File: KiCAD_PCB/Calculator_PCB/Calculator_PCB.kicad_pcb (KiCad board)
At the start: 2 copper layers, 108 parts, among them J1 USB_B_Micro, SW1 SW_SPST, SW10 SW_SPST, SW11 SW_SPST, SW12 SW_SPST, SW13 SW_SPST, SW14 SW_SPST, SW15 SW_SPST, SW16 SW_SPST, SW17 SW_SPST, SW18 SW_SPST, SW19 SW_SPST, SW2 SW_SPST, SW20 SW_SPST, SW21 SW_SPST, SW22 SW_SPST, SW23 SW_SPST, SW24 SW_SPST, SW25 SW_SPST, SW26 SW_SPST, SW27 SW_SPST, SW28 SW_SPST, SW29 SW_SPST, SW3 SW_SPST, SW30 SW_SPST, SW31 SW_SPST, SW32 SW_SPST, SW33 SW_SPST, SW34 SW_SPST, SW35 SW_SPST, SW36 SW_SPST, SW37 SW_SPST, SW38 SW_SPST, SW39 SW_SPST, SW4 SW_SPST, SW40 SW_SPST, SW5 SW_SPST, SW6 SW_SPST, SW7 SW_SPST, SW8 SW_SPST, SW9 SW_SPST, U1 W25Q128JVS, U2 RP2040, U3 NCP1117-3.3_SOT223, Y1 ABLS-12.000MHZ-B4-T

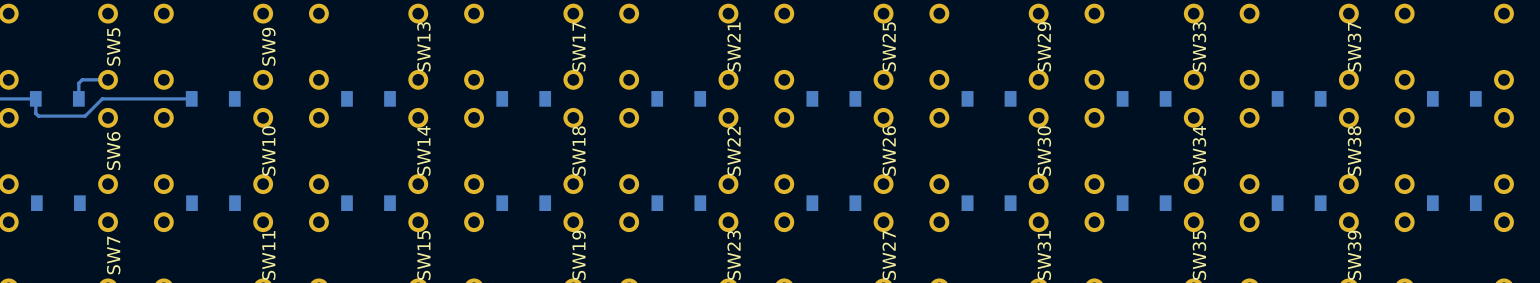
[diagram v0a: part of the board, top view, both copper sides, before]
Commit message: PCB Updates
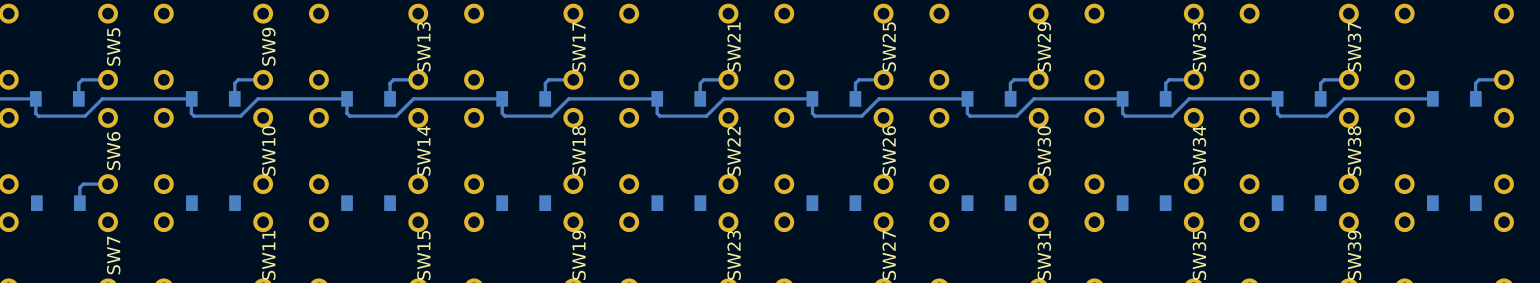
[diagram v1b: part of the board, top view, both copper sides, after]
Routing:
- net /Row0: track 17.6 -> 127.3 mm
- net Net-(D29-Pad2): track 0.00 -> 3.55 mm
- net Net-(D9-Pad2): track 0.00 -> 3.55 mm
- net Net-(D37-Pad2): track 0.00 -> 3.55 mm
- net Net-(D33-Pad2): track 0.00 -> 3.55 mm
- net Net-(D21-Pad2): track 0.00 -> 3.55 mm
- net Net-(D17-Pad2): track 0.00 -> 3.55 mm
- net Net-(D13-Pad2): track 0.00 -> 3.55 mm
- net Net-(D2-Pad2): track 0.00 -> 3.55 mm
- net Net-(D5-Pad2): track 0.00 -> 3.55 mm
- net Net-(D25-Pad2): track 0.00 -> 3.55 mm

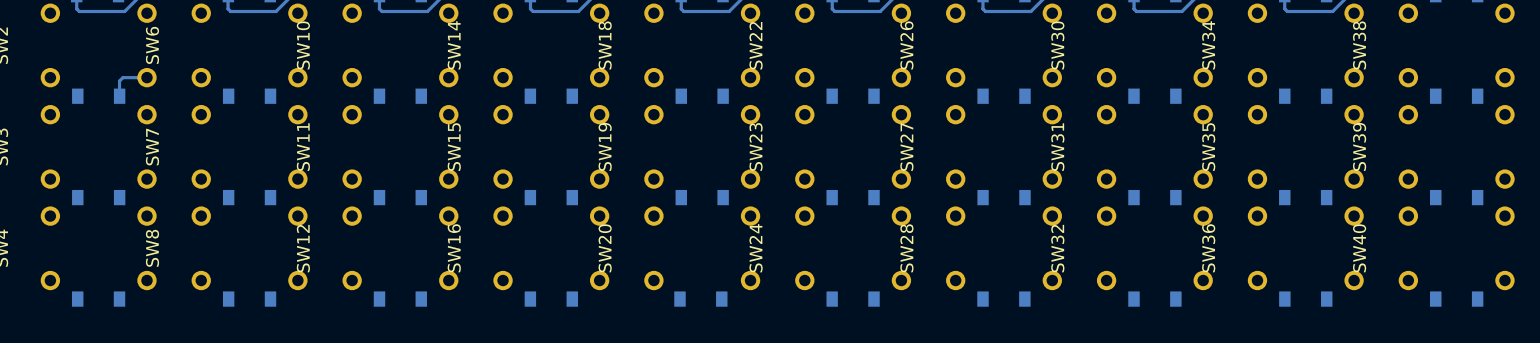
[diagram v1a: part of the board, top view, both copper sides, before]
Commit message: PCB Updates
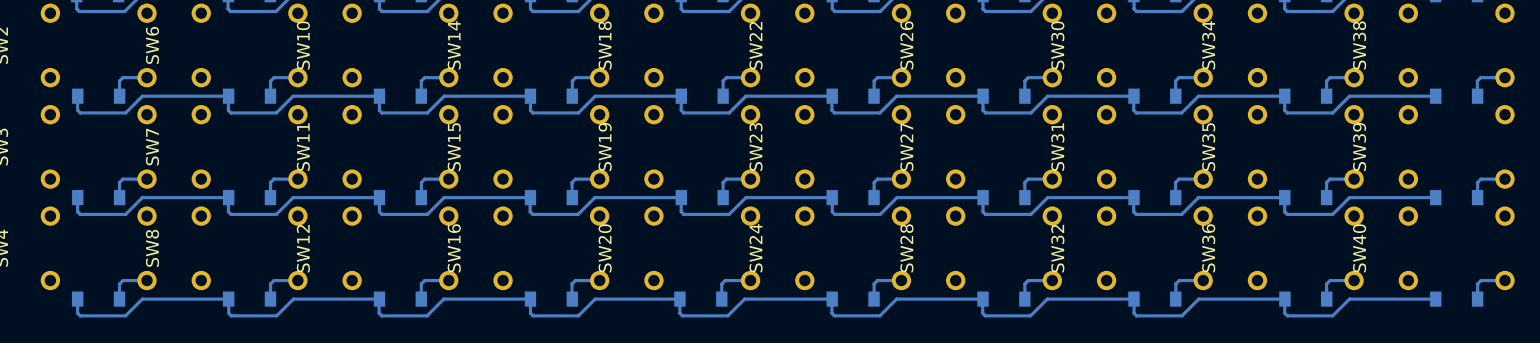
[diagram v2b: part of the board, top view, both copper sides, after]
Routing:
- net /Row3: track 0.00 -> 123.4 mm
- net /Row1: track 0.00 -> 123.4 mm
- net /Row2: track 0.00 -> 123.4 mm
- net Net-(D15-Pad2): track 0.00 -> 3.55 mm
- net Net-(D7-Pad2): track 0.00 -> 3.55 mm
- net Net-(D39-Pad2): track 0.00 -> 3.55 mm
- net Net-(D35-Pad2): track 0.00 -> 3.55 mm
- net Net-(D31-Pad2): track 0.00 -> 3.55 mm
- net Net-(D3-Pad2): track 0.00 -> 3.55 mm
- net Net-(D23-Pad2): track 0.00 -> 3.55 mm
- net Net-(D19-Pad2): track 0.00 -> 3.55 mm
- net Net-(D11-Pad2): track 0.00 -> 3.55 mm
- net Net-(D10-Pad2): track 0.00 -> 3.55 mm
- net Net-(D6-Pad2): track 0.00 -> 3.55 mm
- net Net-(D38-Pad2): track 0.00 -> 3.55 mm
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
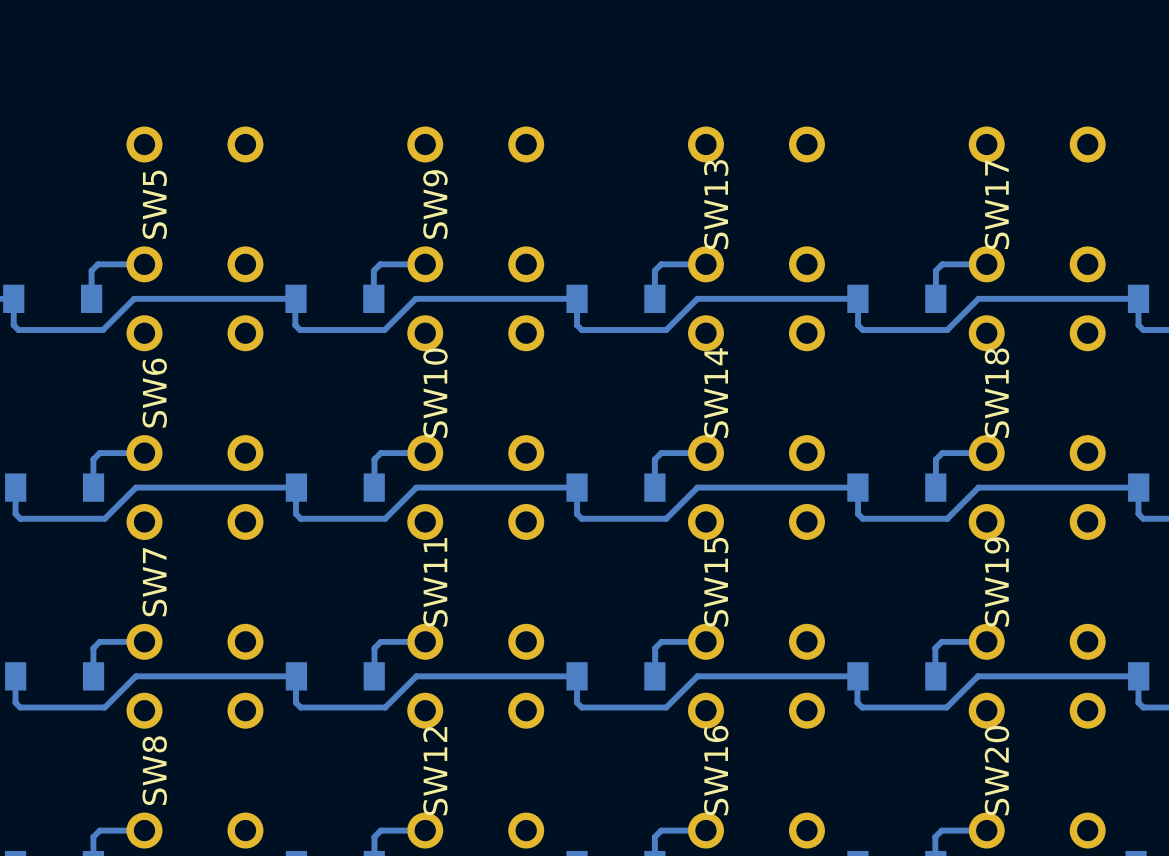
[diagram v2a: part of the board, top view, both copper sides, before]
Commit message: PCB Updates
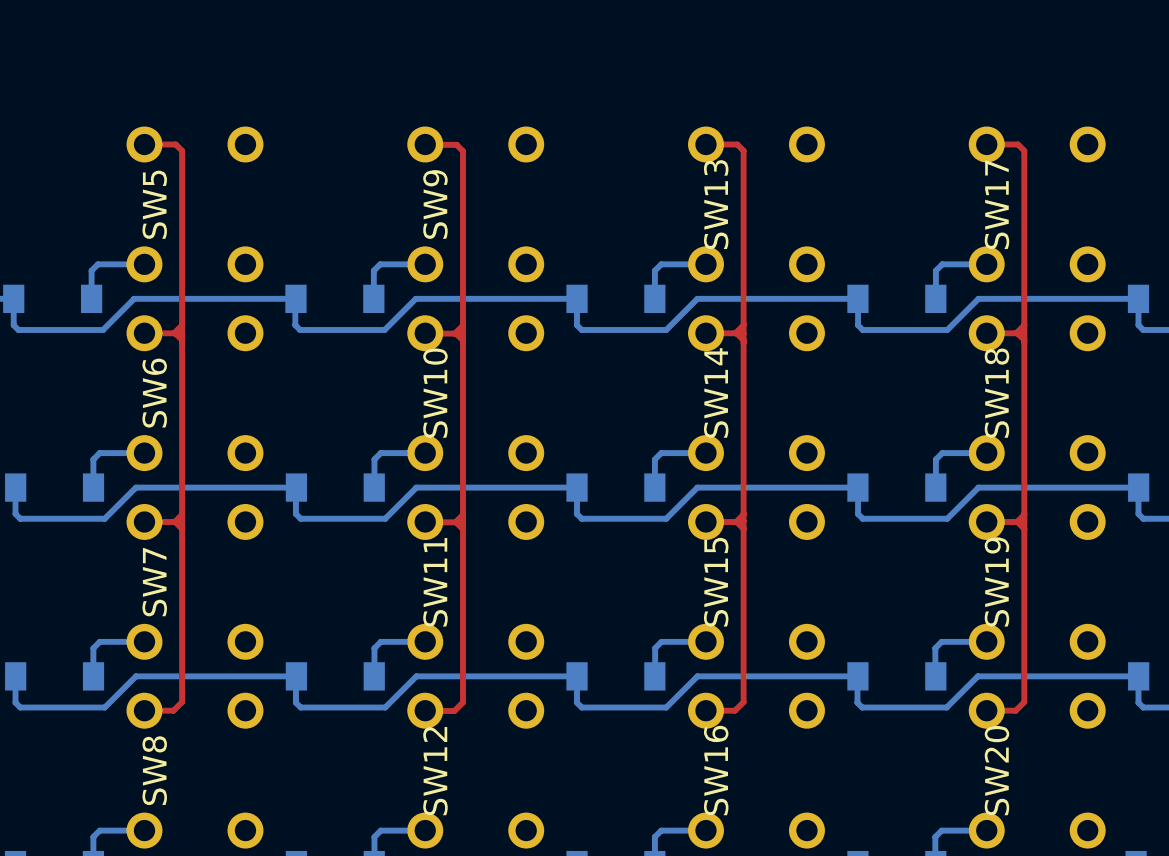
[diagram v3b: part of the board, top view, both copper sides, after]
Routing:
- net /Col0: track 0.00 -> 31.9 mm
- net /Col2: track 0.00 -> 31.8 mm
- net /Col1: track 0.00 -> 31.8 mm
- net /Col3: track 0.00 -> 31.8 mm
